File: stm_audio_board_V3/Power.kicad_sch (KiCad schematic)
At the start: 100 parts, among them J5 Barrel_Jack_MountingPin, U1 IS42S16100H-7TL, U2 OP275, U3 7909, U4 OP275, U5 MIC2920A-3.3WS-TR, U6 7809, U9 MIC2920A-3.3WS-TR

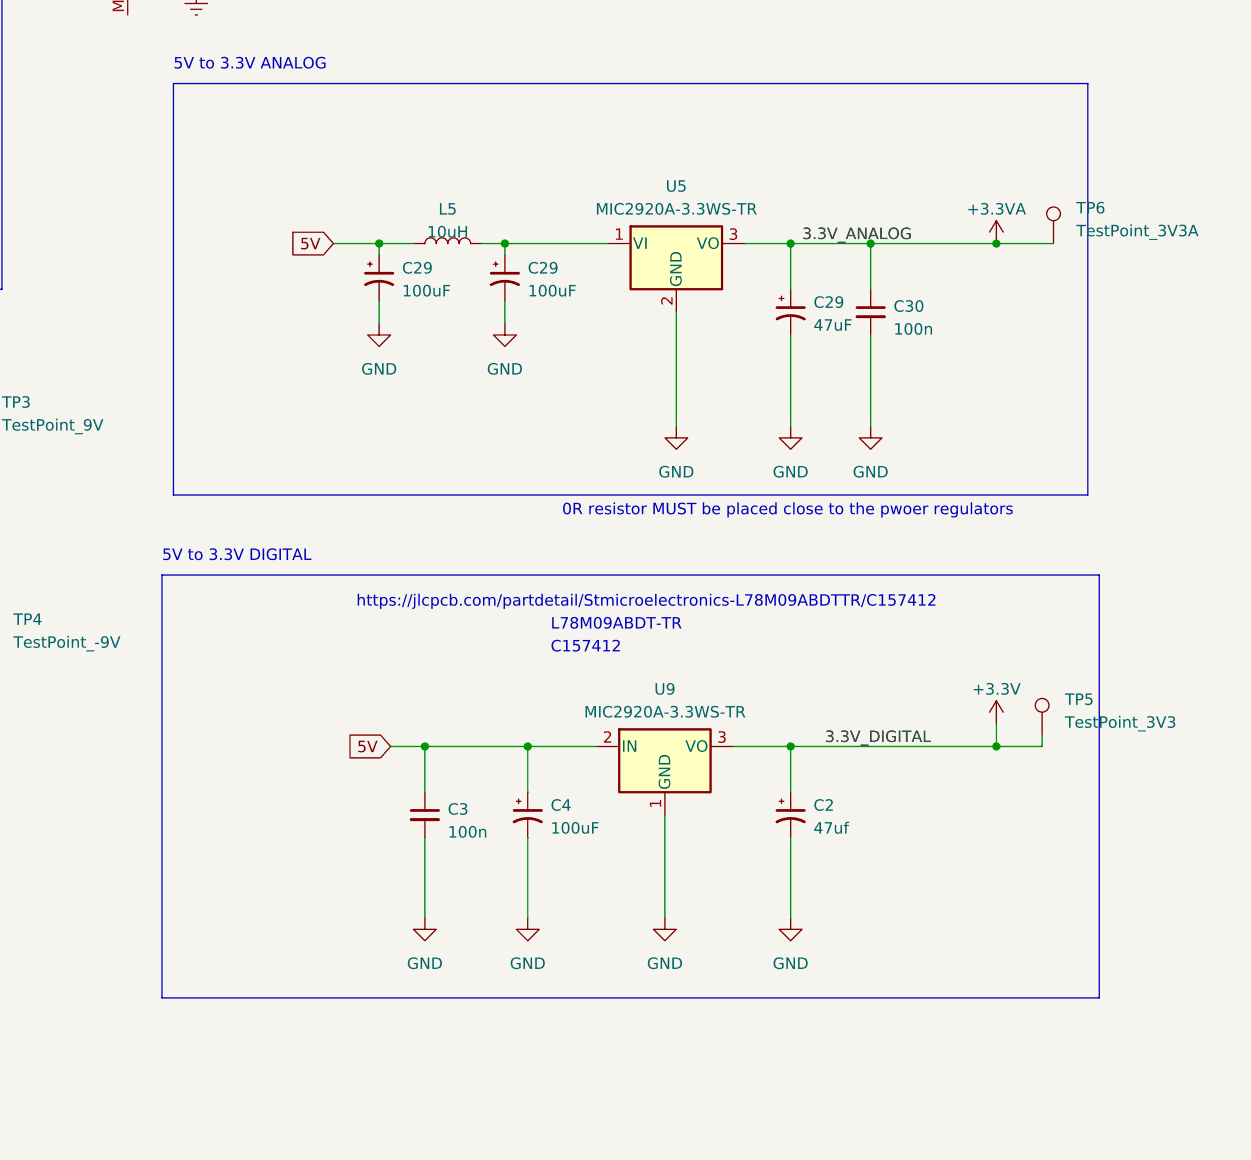
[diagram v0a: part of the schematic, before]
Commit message: minor commit
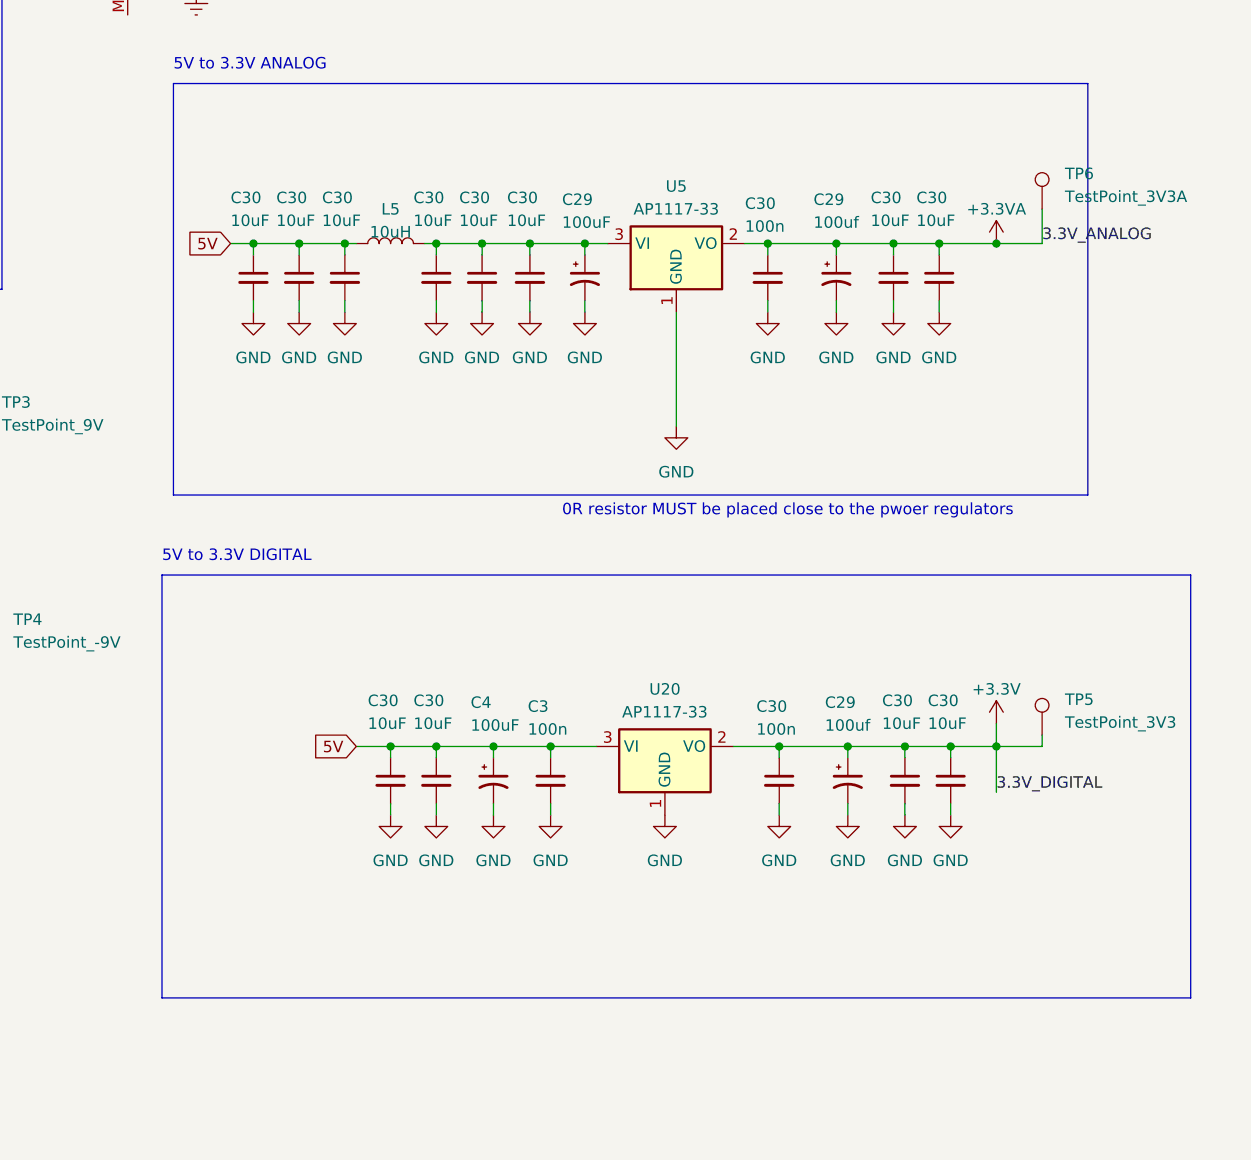
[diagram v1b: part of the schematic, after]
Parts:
- removed C2: 47uf, Capacitor_THT:CP_Radial_D6.3mm_P2.50mm, symbol Device:C_Polarized_Small_US
- removed U5: MIC2920A-3.3WS-TR, Package_TO_SOT_SMD:SOT-223-3_TabPin2, symbol Regulator_Linear:LF33_TO252
- removed U9: MIC2920A-3.3WS-TR, Package_TO_SOT_SMD:SOT-89-3, symbol Regulator_Linear:LF33_TO252
- added C30 (x12): 10uF, Capacitor_SMD:C_1206_3216Metric, symbol Device:C_Small
- added C30: 100n, Capacitor_SMD:C_0603_1608Metric, symbol Device:C_Small
- added U20, U5: AP1117-33, Package_TO_SOT_SMD:SOT-223-3_TabPin2, symbol Regulator_Linear:AP1117-33
- C29: value 100uF -> 100uf
- C29: value 47uF -> 100uf
- U3: JLCPCB (none) -> C8623
- U6: JLCPCB (none) -> C5451665
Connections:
- net +3.3V: now also C29.1, C30.1, C30.1, C30.1, U20.2 (VO)
- net +3.3VA: now also C30.1, C30.1, U5.2 (VO)
- net 5V: now also C30.1, C30.1, C30.1, C30.1, C30.1, U20.3 (VI); no longer C29.1
- net GND: now also C30.2, C30.2, C30.2, C30.2, C30.2, C30.2, C30.2, C30.2, C30.2, C30.2, C30.2, C30.2, C30.2, U20.1 (GND), U5.1 (GND)
- net at C29.1, L5.2: now also C30.1, C30.1, C30.1, U5.3 (VI)
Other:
- note removed: "C157412"
- note removed: "L78M09ABDT-TR"
- note removed: "https://jlcpcb.com/partdetail/Stmicroelectronics-L78M09ABDTTR/C157412"
- moved on the sheet: C29, C3, C30, C4, L5, TP6
